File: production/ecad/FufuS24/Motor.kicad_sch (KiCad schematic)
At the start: 10 parts, among them J5 691137710004, U12 Pololu_DRV8711_Motor_Driver

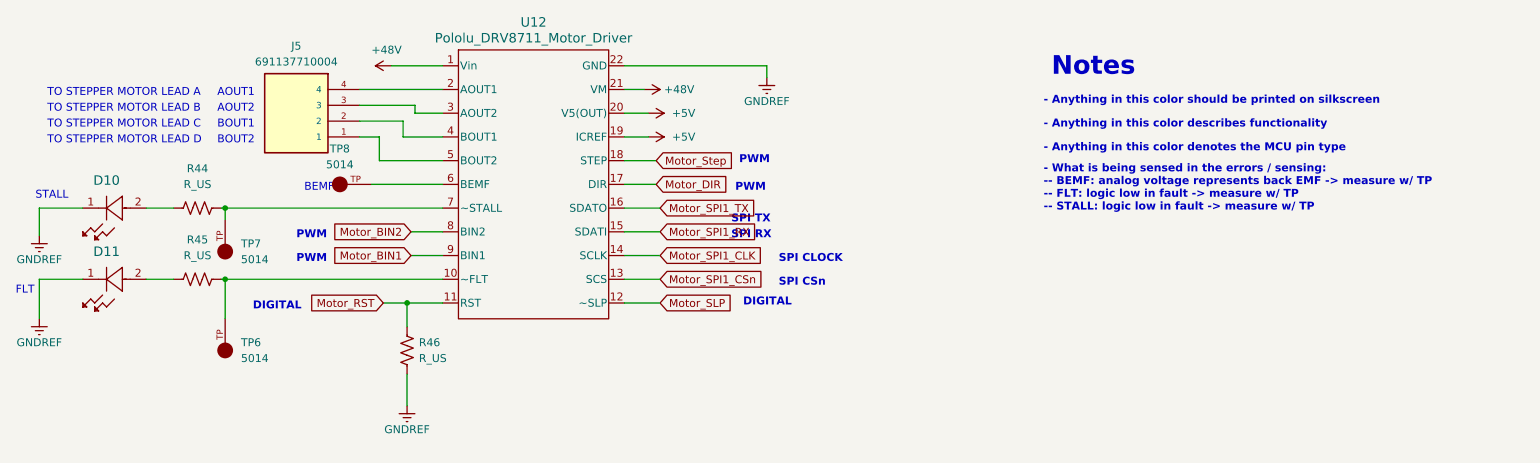
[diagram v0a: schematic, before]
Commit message: i am pulling my hair out
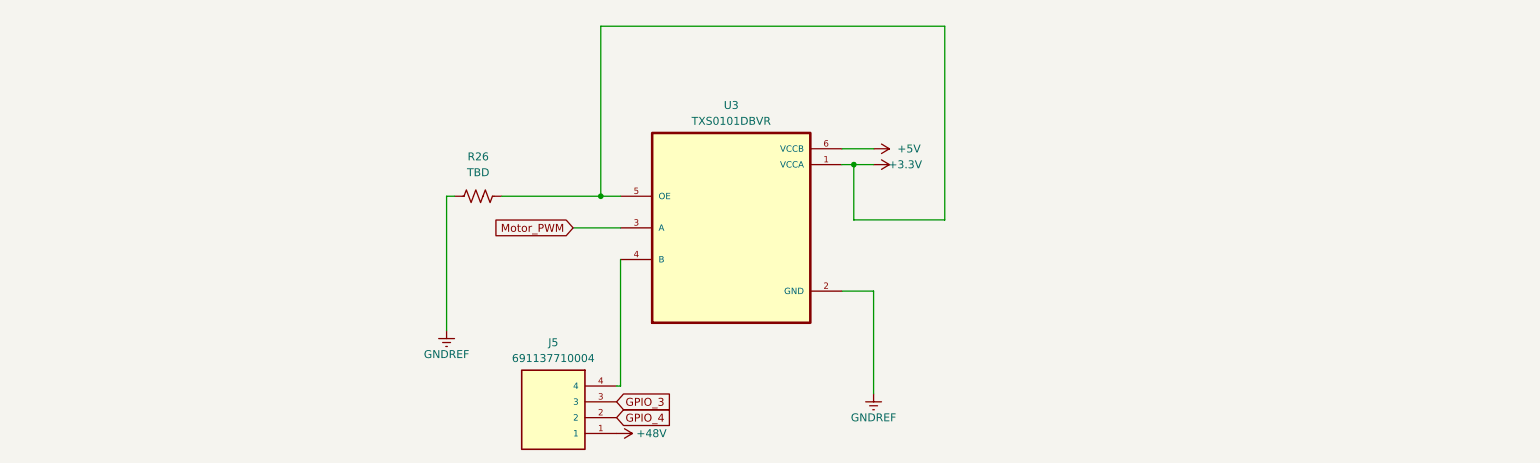
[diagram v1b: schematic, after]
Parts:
- removed D10, D11: 150080GS75000, footprints:LED_GS75000_WRE, symbol 150080GS75000:150080GS75000
- removed R44, R45, R46: R_US, footprints:RESC2012X60N, symbol Device:R_US
- removed TP6, TP7, TP8: 5014, footprints:TP_5014, symbol 5014:5014
- removed U12: Pololu_DRV8711_Motor_Driver, footprints:POLOLU_36v4, symbol POLOLU_35v4:Pololu_DRV8711_Motor_Driver
- added R26: TBD, footprints:RESC2012X60N, symbol Device:R_US
- added U3: TXS0101DBVR, TXS0101DBVR:SOT95P280X145-6N, symbol LevelShifter_Motor:TXS0101DBVR
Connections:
- net +48V: now also J5.1
- net +5V: now also U3.6 (VCCB)
- net GNDREF: now also R26.2, U3.2 (GND)
- net at J5.4: now also U3.4 (B)
- net GPIO_3: now reaches J5.3
- net GPIO_4: now reaches J5.2
- new net +3.3V: R26.1, U3.1 (VCCA), U3.5 (OE)
- new net Motor_PWM: U3.3 (A)
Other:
- note removed: "- Anything in this color denotes the MCU pin type"
- note removed: "- Anything in this color describes functionality"
- note removed: "- Anything in this color should be printed on silkscreen"
- note removed: "- What is being sensed in the errors / sensing: -- BEMF: analog voltage represents back EMF -> measure w/ TP -- FLT: logic low in fault -> measure w/ TP -- STALL: logic low in fault -> measure w/ TP"
- note removed: "AOUT1"
- note removed: "AOUT2"
- note removed: "BEMF"
- note removed: "BOUT1"
- note removed: "BOUT2"
- note removed: "DIGITAL"
- note removed: "FLT"
- note removed: "Notes"
- note removed: "PWM"
- note removed: "SPI CLOCK"
- note removed: "SPI CSn"
- note removed: "SPI RX"
- note removed: "SPI TX"
- note removed: "STALL"
- note removed: "TO STEPPER MOTOR LEAD A"
- note removed: "TO STEPPER MOTOR LEAD B"
- note removed: "TO STEPPER MOTOR LEAD C"
- note removed: "TO STEPPER MOTOR LEAD D"
- moved on the sheet: J5

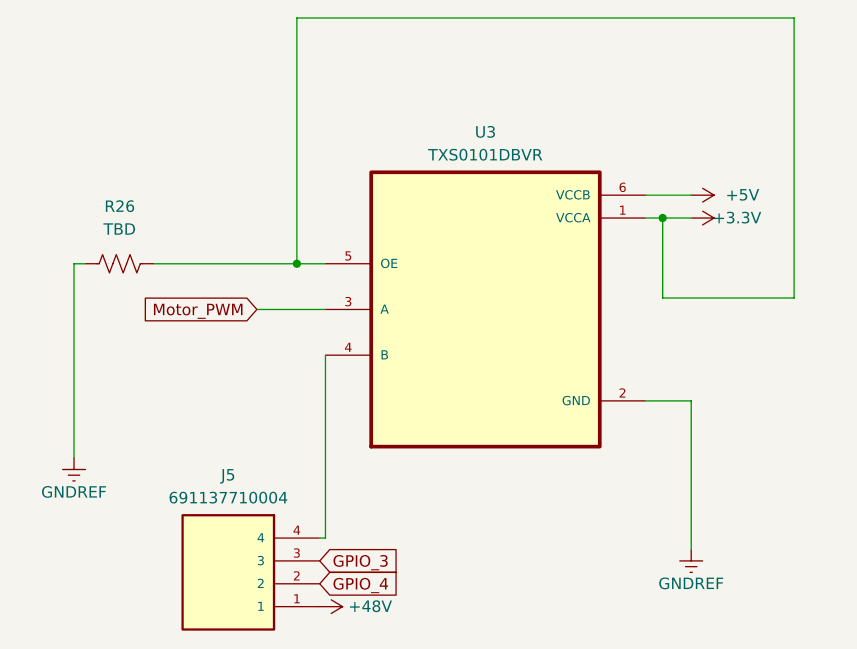
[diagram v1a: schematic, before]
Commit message: changes
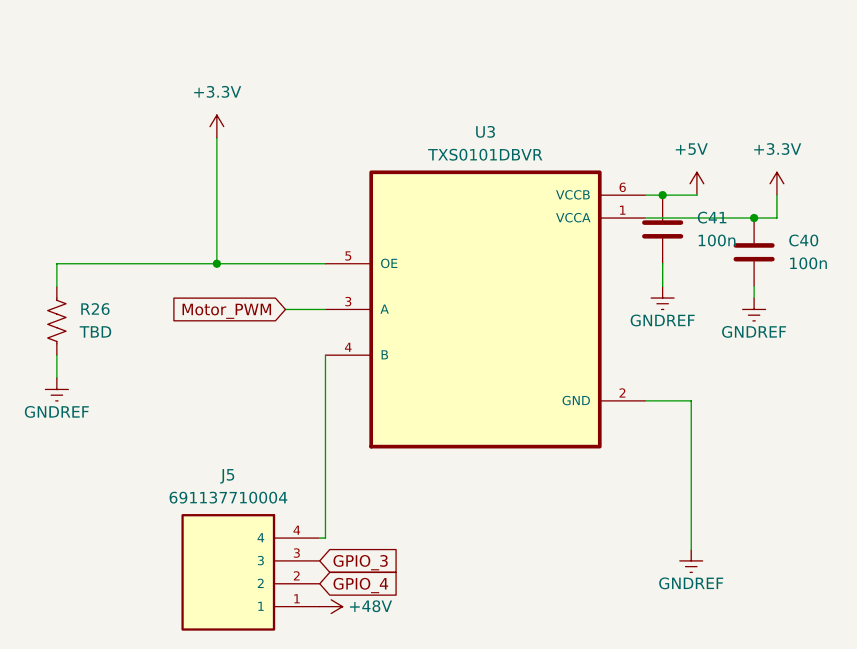
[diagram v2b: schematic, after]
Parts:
- added C40, C41: 100n, footprints:WCAP-CSGP_885012206026, symbol Device:C
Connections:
- net +3.3V: now also C40.1
- net +5V: now also C41.1
- net GNDREF: now also C40.2, C41.2
